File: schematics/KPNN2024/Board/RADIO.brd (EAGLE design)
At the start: 68.2 x 68.2 mm, 16 parts, among them J1 IPX-RADIO, J2 IPX-ANT

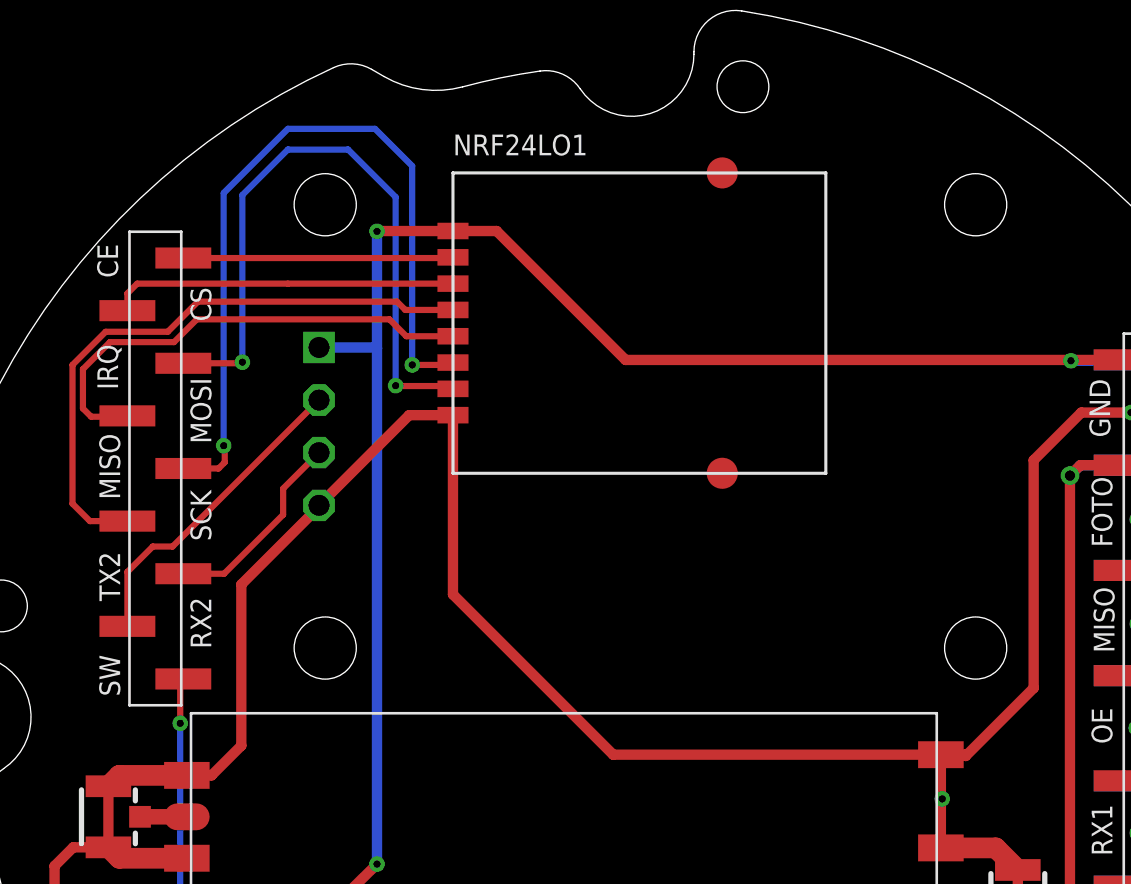
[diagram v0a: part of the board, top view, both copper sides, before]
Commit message: сдклвл платы а мботрен зз
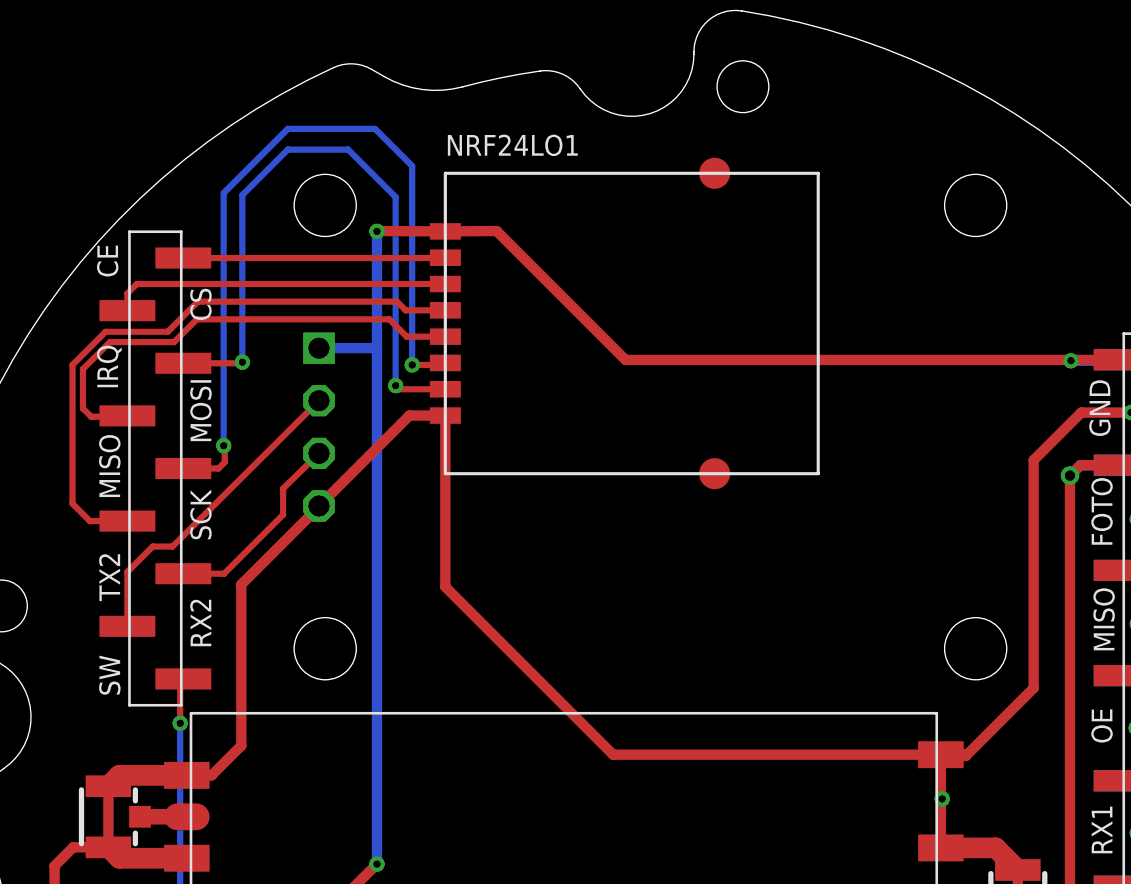
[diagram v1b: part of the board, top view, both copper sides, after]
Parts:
- moved NRF24LO1 0.37 mm to (50.0, 69.0)
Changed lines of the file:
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@@
 <attribute name="VALUE" x="24.5599875" y="48.321015625" size="1" layer="27" font="vector" ratio="15" align="center"/>
 </element>
-<element name="GPS-NEO7M" library="UNKNOWN-2024" package="GPS-NEO7M" value="GPS-NEO7M" x="50.900509375" y="64.0324625" smashed="yes" rot="MR270">
-<attribute name="NAME" x="61.5324625" y="77.099490625" size="1" layer="28" font="vector" ratio="15" rot="MR0"/>
-</element>
-<element name="NRF24LO1" library="UNKNOWN-2024" package="NRF24L01_ML01SP4" value="NRF24L01_ML01SP4" x="50.36748125" y="69.018953125" smashed="yes">
-<attribute name="NAME" x="41.36748125" y="77.118953125" size="1" layer="25" font="vector" ratio="15"/>
+<element name="GPS-NEO7M" library="UNKNOWN-2024" package="GPS-NEO7M" value="GPS-NEO7M" x="50.9" y="64" smashed="yes" rot="MR270">
+<attribute name="NAME" x="61.531953125" y="77.067028125" size="1" layer="28" font="vector" ratio="15" rot="MR0"/>
+</element>
+<element name="NRF24LO1" library="UNKNOWN-2024" package="NRF24L01_ML01SP4" value="NRF24L01_ML01SP4" x="50" y="69" smashed="yes">
+<attribute name="NAME" x="41" y="77.1" size="1" layer="25" font="vector" ratio="15"/>
 </element>
 <element name="XQ-02A" library="UNKNOWN-2024" package="XQ-02A" value="XQ-02A" x="46.721015625" y="37.18434375" smashed="yes" rot="R180">
@@
 <wire x1="29.714175" y1="47.18434375" x2="31.15" y2="48.62016875" width="0.5" layer="1"/>
 <wire x1="31.15" y1="56.4" x2="31.15" y2="48.62016875" width="0.5" layer="1"/>
-<wire x1="34.900509375" y1="60.2224625" x2="34.900509375" y2="60.150509375" width="0.5" layer="1"/>
+<wire x1="34.9" y1="60.19" x2="34.900509375" y2="60.150509375" width="0.5" layer="1"/>
 <wire x1="34.900509375" y1="60.150509375" x2="31.15" y2="56.4" width="0.5" layer="1"/>
-<wire x1="34.900509375" y1="60.2224625" x2="39.252" y2="64.573953125" width="0.5" layer="1"/>
-<wire x1="39.252" y1="64.573953125" x2="41.36748125" y2="64.573953125" width="0.5" layer="1"/>
-<wire x1="41.36748125" y1="64.573953125" x2="41.36748125" y2="55.9168625" width="0.5" layer="1"/>
-<wire x1="41.36748125" y1="55.9168625" x2="49.1" y2="48.18434375" width="0.5" layer="1"/>
+<wire x1="41" y1="56.28434375" x2="49.1" y2="48.18434375" width="0.5" layer="1"/>
 <wire x1="49.1" y1="48.18434375" x2="64.921015625" y2="48.18434375" width="0.5" layer="1"/>
 <wire x1="64.921015625" y1="48.18434375" x2="64.921015625" y2="43.68434375" width="0.5" layer="1"/>
@@
 <wire x1="24.734015625" y1="46.66034375" x2="25.258015625" y2="47.18434375" width="1" layer="1"/>
 <wire x1="25.258015625" y1="47.18434375" x2="28.521015625" y2="47.18434375" width="1" layer="1"/>
+<wire x1="41" y1="64.555" x2="41" y2="56.28434375" width="0.5" layer="1"/>
+<wire x1="34.9" y1="60.19" x2="39.265" y2="64.555" width="0.5" layer="1"/>
+<wire x1="39.265" y1="64.555" x2="41" y2="64.555" width="0.5" layer="1"/>
 </signal>
 <signal name="3V3">
@@
 <wire x1="31.08238125" y1="36.38238125" x2="37.7" y2="42.9" width="0.5" layer="1"/>
 <via x="37.7" y="42.9" extent="1-16" drill="0.35"/>
-<wire x1="41.36748125" y1="73.463953125" x2="37.736046875" y2="73.463953125" width="0.5" layer="1"/>
+<wire x1="41" y1="73.445" x2="37.736046875" y2="73.463953125" width="0.5" layer="1"/>
 <wire x1="37.736046875" y1="73.463953125" x2="37.7" y2="73.5" width="0.5" layer="1"/>
 <wire x1="37.7" y1="73.5" x2="37.7" y2="73.45" width="0.5" layer="1"/>
 <via x="37.7" y="73.45" extent="1-16" drill="0.35"/>
-<wire x1="41.36748125" y1="73.463953125" x2="43.476046875" y2="73.463953125" width="0.5" layer="1"/>
+<wire x1="41" y1="73.445" x2="43.476046875" y2="73.463953125" width="0.5" layer="1"/>
 <wire x1="43.476046875" y1="73.463953125" x2="49.7" y2="67.24" width="0.5" layer="1"/>
 <wire x1="71.16" y1="67.24" x2="71.2" y2="67.2" width="0.5" layer="1"/>
@@
 <wire x1="37.7" y1="42.9" x2="37.7" y2="67.8" width="0.5" layer="16"/>
 <wire x1="37.7" y1="67.8" x2="37.7" y2="73.45" width="0.5" layer="16"/>
-<wire x1="34.900509375" y1="67.8424625" x2="37.6575375" y2="67.8424625" width="0.5" layer="16"/>
-<wire x1="37.6575375" y1="67.8424625" x2="37.7" y2="67.8" width="0.5" layer="16"/>
+<wire x1="34.9" y1="67.81" x2="37.69" y2="67.81" width="0.5" layer="16"/>
+<wire x1="37.69" y1="67.81" x2="37.7" y2="67.8" width="0.5" layer="16"/>
 </signal>
 <signal name="5V">
@@
 <contactref element="NRF24LO1" pad="P$2"/>
 <wire x1="28.35" y1="72.16" x2="41.333528125" y2="72.16" width="0.3" layer="1"/>
-<wire x1="41.333528125" y1="72.16" x2="41.36748125" y2="72.193953125" width="0.3" layer="1"/>
+<wire x1="41.333528125" y1="72.16" x2="41" y2="72.175" width="0.3" layer="1"/>
 </signal>
 <signal name="CS_RADIO">
@@
 <contactref element="NRF24LO1" pad="P$3"/>
 <wire x1="25.65" y1="69.62" x2="25.65" y2="70.45" width="0.3" layer="1"/>
-<wire x1="25.65" y1="70.45" x2="26.123953125" y2="70.923953125" width="0.3" layer="1"/>
-<wire x1="26.123953125" y1="70.923953125" x2="33.4" y2="70.923953125" width="0.3" layer="1"/>
-<wire x1="33.4" y1="70.923953125" x2="41.36748125" y2="70.923953125" width="0.3" layer="1"/>
+<wire x1="25.65" y1="70.45" x2="26.105" y2="70.905" width="0.3" layer="1"/>
+<wire x1="26.105" y1="70.905" x2="41" y2="70.905" width="0.3" layer="1"/>
 </signal>
 <signal name="IRQ_RADIO">
 <contactref element="U$7" pad="3"/>
 <contactref element="NRF24LO1" pad="P$7"/>
-<wire x1="41.36748125" y1="65.843953125" x2="41.23090625" y2="65.980528125" width="0.3" layer="1"/>
-<wire x1="41.23090625" y1="65.980528125" x2="38.619471875" y2="65.980528125" width="0.3" layer="1"/>
-<wire x1="38.619471875" y1="65.980528125" x2="38.6" y2="66" width="0.3" layer="1"/>
 <via x="38.6" y="66" extent="1-16" drill="0.35"/>
 <wire x1="38.6" y1="75.10326875" x2="38.6" y2="66" width="0.3" layer="16"/>
@@
 <wire x1="38.6" y1="75.10326875" x2="36.30480625" y2="77.3984625" width="0.3" layer="16"/>
 <wire x1="33.3984625" y1="77.3984625" x2="31.2006375" y2="75.2006375" width="0.3" layer="16"/>
+<wire x1="38.6" y1="66" x2="38.775" y2="65.825" width="0.3" layer="1"/>
+<wire x1="38.775" y1="65.825" x2="41" y2="65.825" width="0.3" layer="1"/>
 </signal>
 <signal name="MOSI_RADIO">
 <contactref element="U$7" pad="4"/>
 <contactref element="NRF24LO1" pad="P$5"/>
-<wire x1="41.36748125" y1="68.383953125" x2="39.116046875" y2="68.383953125" width="0.3" layer="1"/>
-<wire x1="39.116046875" y1="68.383953125" x2="38.3" y2="69.2" width="0.3" layer="1"/>
-<wire x1="38.3" y1="69.2" x2="29" y2="69.2" width="0.3" layer="1"/>
+<wire x1="29" y1="69.2" x2="38.3" y2="69.2" width="0.3" layer="1"/>
 <wire x1="24.8071125" y1="68.1" x2="23.50355625" y2="66.79644375" width="0.3" layer="1"/>
 <wire x1="23.50355625" y1="66.79644375" x2="23.50355625" y2="64.89644375" width="0.3" layer="1"/>
@@
 <wire x1="29" y1="69.2" x2="27.9" y2="68.1" width="0.3" layer="1"/>
 <wire x1="27.9" y1="68.1" x2="24.8071125" y2="68.1" width="0.3" layer="1"/>
+<wire x1="39.135" y1="68.365" x2="41" y2="68.365" width="0.3" layer="1"/>
+<wire x1="38.3" y1="69.2" x2="39.135" y2="68.365" width="0.3" layer="1"/>
 </signal>
 <signal name="MISO_RADIO">
@@
 <wire x1="30.35" y1="62.3" x2="30.05" y2="62" width="0.3" layer="1"/>
 <wire x1="28.35" y1="62" x2="30.05" y2="62" width="0.3" layer="1"/>
-<wire x1="41.36748125" y1="67.113953125" x2="41.253528125" y2="67" width="0.3" layer="1"/>
-<wire x1="41.253528125" y1="67" x2="39.4" y2="67" width="0.3" layer="1"/>
 <via x="39.4" y="67" extent="1-16" drill="0.35"/>
 <wire x1="39.4" y1="76.6" x2="39.4" y2="67" width="0.3" layer="16"/>
@@
 <wire x1="39.4" y1="76.6" x2="37.6015375" y2="78.3984625" width="0.3" layer="16"/>
 <wire x1="33.3984625" y1="78.3984625" x2="30.3" y2="75.3" width="0.3" layer="16"/>
+<wire x1="39.4" y1="67" x2="40.905" y2="67" width="0.3" layer="1"/>
+<wire x1="40.905" y1="67" x2="41" y2="67.095" width="0.3" layer="1"/>
 </signal>
 <signal name="SCK_RADIO">
@@
 <wire x1="23.84" y1="59.46" x2="23" y2="60.3" width="0.3" layer="1"/>
 <wire x1="23" y1="67" x2="23" y2="60.3" width="0.3" layer="1"/>
-<wire x1="41.36748125" y1="69.653953125" x2="39.06748125" y2="69.653953125" width="0.3" layer="1"/>
-<wire x1="39.06748125" y1="69.653953125" x2="38.66748125" y2="70.053953125" width="0.3" layer="1"/>
-<wire x1="38.66748125" y1="70.053953125" x2="29.053953125" y2="70.053953125" width="0.3" layer="1"/>
+<wire x1="29.053953125" y1="70.053953125" x2="38.66748125" y2="70.053953125" width="0.3" layer="1"/>
 <wire x1="29.053953125" y1="70.053953125" x2="27.6" y2="68.6" width="0.3" layer="1"/>
 <wire x1="27.6" y1="68.6" x2="24.6" y2="68.6" width="0.3" layer="1"/>
 <wire x1="24.6" y1="68.6" x2="23" y2="67" width="0.3" layer="1"/>
+<wire x1="39.086434375" y1="69.635" x2="41" y2="69.635" width="0.3" layer="1"/>
+<wire x1="38.66748125" y1="70.053953125" x2="39.086434375" y2="69.635" width="0.3" layer="1"/>
 </signal>
 <signal name="TX2_GPS">
 <contactref element="U$7" pad="7"/>
 <contactref element="GPS-NEO7M" pad="P$3"/>
-<wire x1="33.169021875" y1="61.030975" x2="34.900509375" y2="62.7624625" width="0.3" layer="1"/>
+<wire x1="33.169021875" y1="61.030975" x2="34.9" y2="62.73" width="0.3" layer="1"/>
 <wire x1="28.35" y1="56.92" x2="30.32" y2="56.92" width="0.3" layer="1"/>
 <wire x1="33.169021875" y1="59.769021875" x2="33.169021875" y2="61.030975" width="0.3" layer="1"/>
@@
 <wire x1="25.65" y1="54.38" x2="25.65" y2="57.00765625" width="0.3" layer="1"/>
 <wire x1="25.65" y1="57.00765625" x2="26.87474375" y2="58.2324" width="0.3" layer="1"/>
-<wire x1="27.830446875" y1="58.2324" x2="34.900509375" y2="65.3024625" width="0.3" layer="1"/>
+<wire x1="27.830446875" y1="58.2324" x2="34.9" y2="65.27" width="0.3" layer="1"/>
 </signal>
 <signal name="SW_WMP">
